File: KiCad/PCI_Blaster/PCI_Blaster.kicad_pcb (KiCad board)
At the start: 2 copper layers, 79.2 x 26.5 mm, 11 parts, among them J1 Bus_PCI_32bit_5V

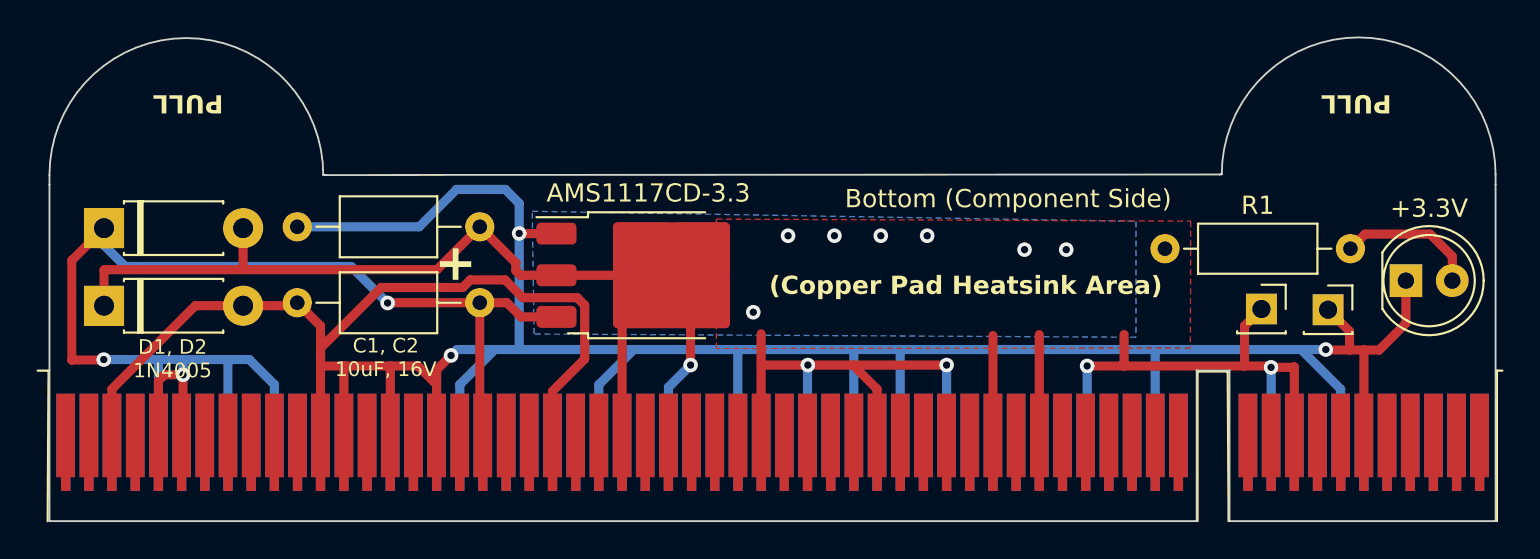
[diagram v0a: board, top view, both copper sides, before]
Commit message: redo pcb layout
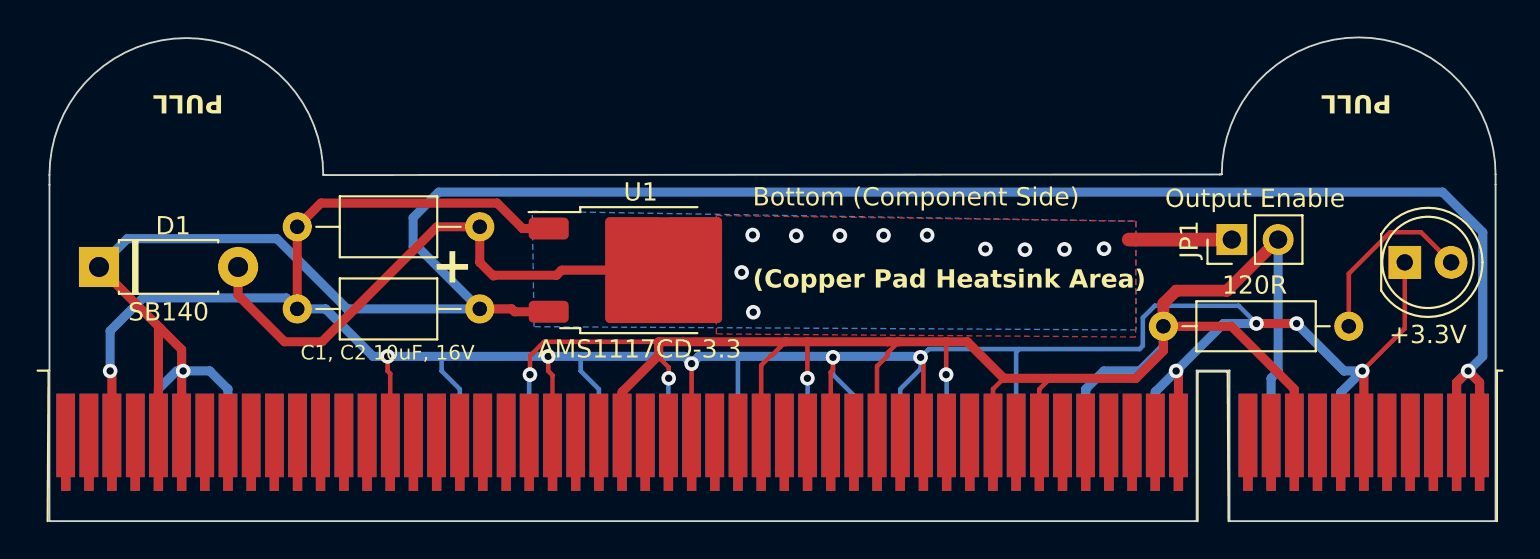
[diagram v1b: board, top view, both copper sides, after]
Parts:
- removed AMS1117CD-3.3: AMS1117CD-3.3, Package_TO_SOT_SMD:TO-252-3_TabPin2
- removed D2: 1N4005, Diode_THT:D_DO-41_SOD81_P7.62mm_Horizontal
- removed REF**: OSHW-Logo2_9.8x8mm_SilkScreen, Symbol:OSHW-Logo2_9.8x8mm_SilkScreen
- removed TP1: +3.3V, Connector_PinSocket_2.54mm:PinSocket_1x01_P2.54mm_Vertical
- removed TP2: GND, Connector_PinSocket_2.54mm:PinSocket_1x01_P2.54mm_Vertical
- added JP1: Output Enable, Connector_PinHeader_2.54mm:PinHeader_1x02_P2.54mm_Vertical, F.Cu at (179.2, 98.0)
- added U1: AMS1117CD-3.3, Package_TO_SOT_SMD:TO-252-2, F.Cu at (146.9, 99.7)
- D1: value 1N4005 -> SB140
- LED1: renamed from +3.3V; value +3,3V -> +3.3V
- moved R1 4.25 mm to (175.5, 102.8)
- moved D1 2.14 mm to (117.2, 99.5)
- moved LED1 1.00 mm to (188.7, 99.2)
- moved C1 0.34 mm to (138.1, 101.8)
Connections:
- C2 pad 1: +3.3V -> /V_OUT
- D1 pad 2: +3.3V -> /V_OUT
- J1 pad A10: +5V -> unconnected-(J1-+5V-PadA10)
- J1 pad A12: GND -> unconnected-(J1-GND-PadA12)
- J1 pad A13: GND -> unconnected-(J1-GND-PadA13)
- J1 pad A16: +5V -> unconnected-(J1-+5V-PadA16)
- J1 pad A42: unconnected-(J1-GND-PadA42) -> GND
- J1 pad A59: +5V -> unconnected-(J1-+5V-PadA59)
- J1 pad B12: GND -> unconnected-(J1-GND-PadB12)
- J1 pad B13: GND -> unconnected-(J1-GND-PadB13)
- J1 pad B17: GND -> unconnected-(J1-GND-PadB17)
- J1 pad B19: +5V -> unconnected-(J1-+5V-PadB19)
- J1 pad B46: GND -> unconnected-(J1-GND-PadB46)
- J1 pad B59: +5V -> unconnected-(J1-+5V-PadB59)
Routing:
- net +5V: track 74.1 -> 143.6 mm, vias 3 -> 2
- net /V_OUT: track 0.00 -> 36.6 mm, vias 0 -> 11
- net GND: track 188.5 -> 176.6 mm, vias 3 -> 10
- net Net-(LED1-A): track 7.75 -> 10.1 mm
- net +3.3V: track 122.4 -> 122.6 mm, vias 12 -> 4
- added copper zone on B.Cu, net /V_OUT
- added copper zone on F.Cu, net /V_OUT
- removed copper zone on B.Cu, net +3.3V
- removed copper zone on F.Cu, net +3.3V
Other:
- board text added: "JLCJLCJLCJLC"
- board text removed: "D1, D2 1N4005"
